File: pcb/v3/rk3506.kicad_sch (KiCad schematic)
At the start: 17 parts, among them J1 TestPoint, J15 TestPoint, J2 Conn_01x03, J3 TestPoint, U1 SOM3562_18

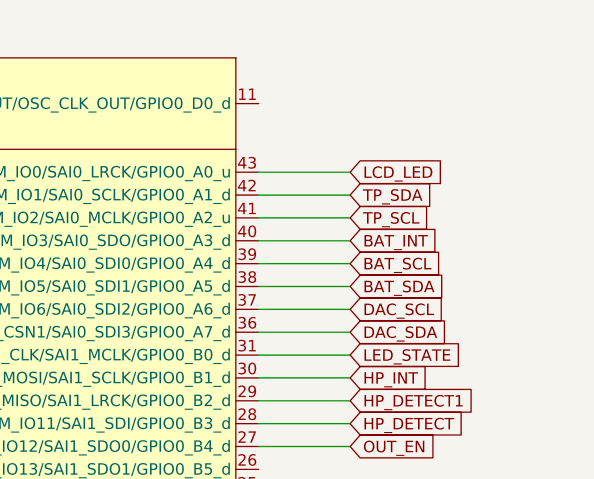
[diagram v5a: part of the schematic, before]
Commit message: 123
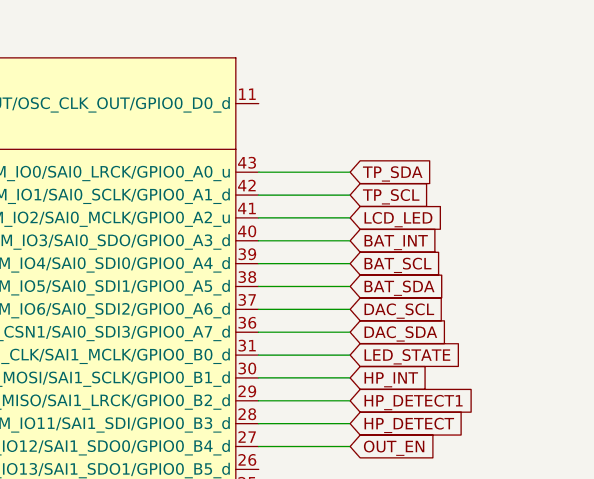
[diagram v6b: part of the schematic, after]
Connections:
- net LCD_LED: now also U1.41 (RM_IO2/SAI0_MCLK/GPIO0_A2_u); no longer U1.43 (RM_IO0/SAI0_LRCK/GPIO0_A0_u)
- net TP_SCL: now also U1.42 (RM_IO1/SAI0_SCLK/GPIO0_A1_d); no longer U1.41 (RM_IO2/SAI0_MCLK/GPIO0_A2_u)
- net TP_SDA: now also U1.43 (RM_IO0/SAI0_LRCK/GPIO0_A0_u); no longer U1.42 (RM_IO1/SAI0_SCLK/GPIO0_A1_d)
